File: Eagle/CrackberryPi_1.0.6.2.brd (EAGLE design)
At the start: 85 x 96 mm, 154 parts, among them IC1 REG1117, IC2 24C02CSM, Q1 IRLML5203, Q4 IRLML5203, Q5 32.768, T1 BC847, T2 BC847, T5 BC847, T6 BC847, T7 BC847, X3 C-GRID-03-70543, X5 FH12-50S-0.5SH

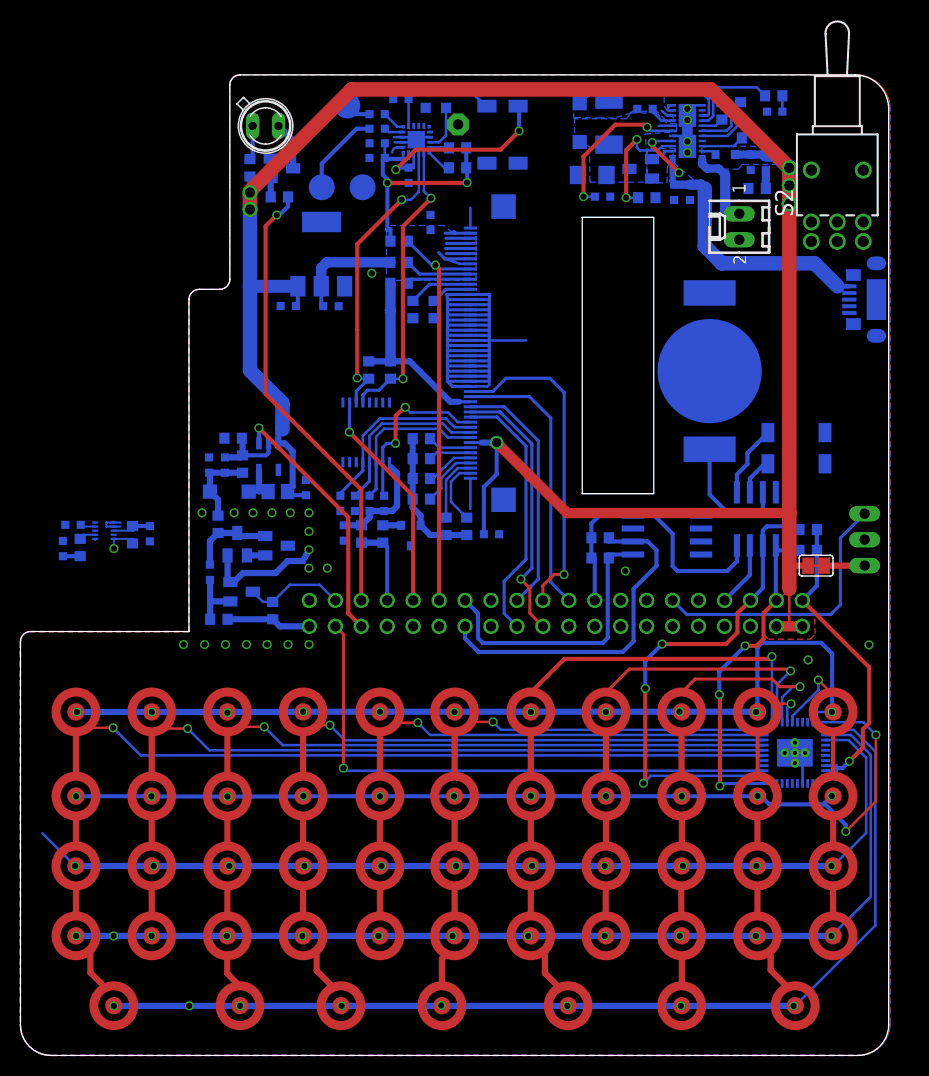
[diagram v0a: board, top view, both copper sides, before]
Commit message: lots of updates
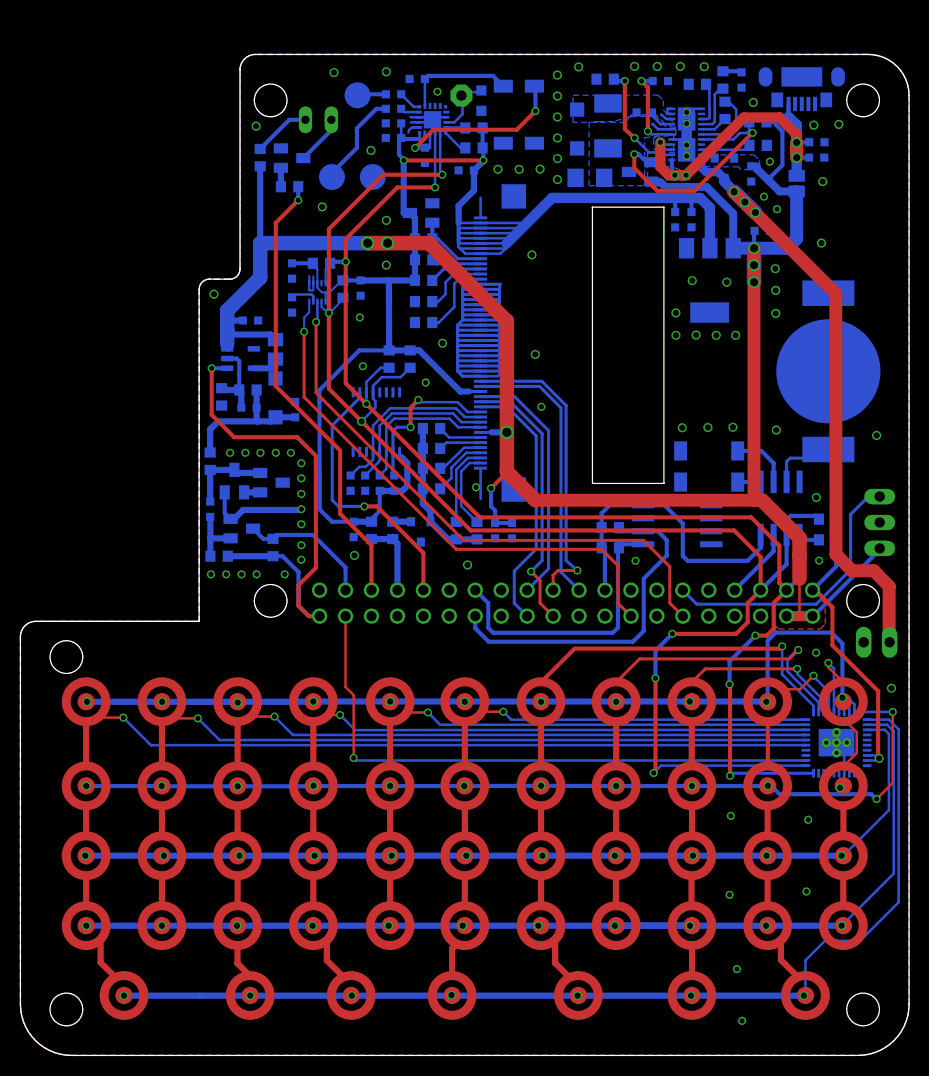
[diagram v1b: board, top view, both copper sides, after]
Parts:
- removed LED1: (no value), led:CHIP-LED0603
- removed R30: 30, rcl:R0603
- removed S2: TL49WO, switch:TL4XWO
- removed SJ2: (no value), jumper:SJ
- added C22: 100nF, rcl:C0603
- added C23: 1mf, rcl:C0603
- added SJ1: (no value), jumper:SJ
- added U$3: RESETMONITOR, MAX803:SOT23
- moved C13 47.0 mm to (72.6, 80.7), turned to 180 degrees
- moved BATTERY 42.8 mm to (83.8, 40.5), flipped to the bottom, turned to 180 degrees
- moved C30 38.7 mm to (33.3, 75.1), turned to 270 degrees
- moved IC1 38.1 mm to (67.5, 75.9), turned to 180 degrees
- moved C14 36.3 mm to (65.7, 81.8), turned to 270 degrees
- moved R34 36.1 mm to (31.6, 75.0), turned to 90 degrees
- moved R33 32.4 mm to (29.5, 77.5), turned to 0 degrees
- moved U$13 31.3 mm to (29.1, 74.7), turned to 90 degrees
- moved C32 30.4 mm to (26.6, 73.5), turned to 270 degrees
- moved C31 29.3 mm to (26.6, 76.8)
- moved C1 24.0 mm to (64.1, 81.8), turned to 270 degrees
- moved U$9 23.0 mm to (76.5, 95.8), turned to 180 degrees
- moved C6 17.2 mm to (22.5, 72.0), turned to 180 degrees
- moved C5 14.8 mm to (78.0, 89.4), turned to 180 degrees
- moved L1 13.9 mm to (25.0, 69.1), turned to 270 degrees
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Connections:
- removed net EMITTER: T1.2
- removed net N$11: LED1.C, R30.2
- removed net STEPUP_ENABLE: U$11.P$36, U$2.1
- new net GPIO16: U$11.P$36
- new net GPIO5: U$11.P$29
- net +3V3: now also C22.1, U$3.3
- net +5V: now also C23.1, SJ1.2; no longer LED1.A, SJ2.1, SJ2.2
- net DISPLAY_RESET: now also U$3.2; no longer U$11.P$29
- net GND: now also C22.2, C23.2, T1.2, U$3.1; no longer R30.1
- net IN: now also SJ1.1
- net RANDOM_POWER: now also U$2.1
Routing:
- net +3V3: track 91.0 -> 180.5 mm
- net SCL_3V3: track 79.9 -> 150.1 mm, vias 5 -> 6
- net SDA_3V3: track 68.1 -> 130.1 mm
- net ACC_INT1: track 0.00 -> 56.2 mm, vias 0 -> 1
- net BAT: track 8.46 -> 61.1 mm, vias 0 -> 3
- net ACC_INT2: track 0.00 -> 52.6 mm, vias 0 -> 1
- net RANDOM_POWER: track 8.30 -> 49.4 mm, vias 0 -> 1
- net DISPLAY_RESET: track 40.2 -> 7.11 mm, vias 1 -> 0
- net STEPUP_ENABLE: track 25.1 -> 0.00 mm, vias 1 -> 0
- net HVPR: track 4.60 -> 24.6 mm, vias 0 -> 2
- net +5V: track 221.1 -> 201.7 mm, vias 6 -> 7
- net GND: track 137.3 -> 128.9 mm, vias 25 -> 88
- net N$7: track 15.3 -> 8.74 mm
- net +15V: track 7.84 -> 14.2 mm
- net VBAT+: track 12.3 -> 6.62 mm
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- removed copper zone on layer 16, net +3V3
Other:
- board size 85 x 96 mm -> 87 x 98 mm
